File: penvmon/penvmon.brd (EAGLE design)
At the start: 91.9 x 100 mm, 19 parts, among them IC2 7805TV, U1 ZC563900

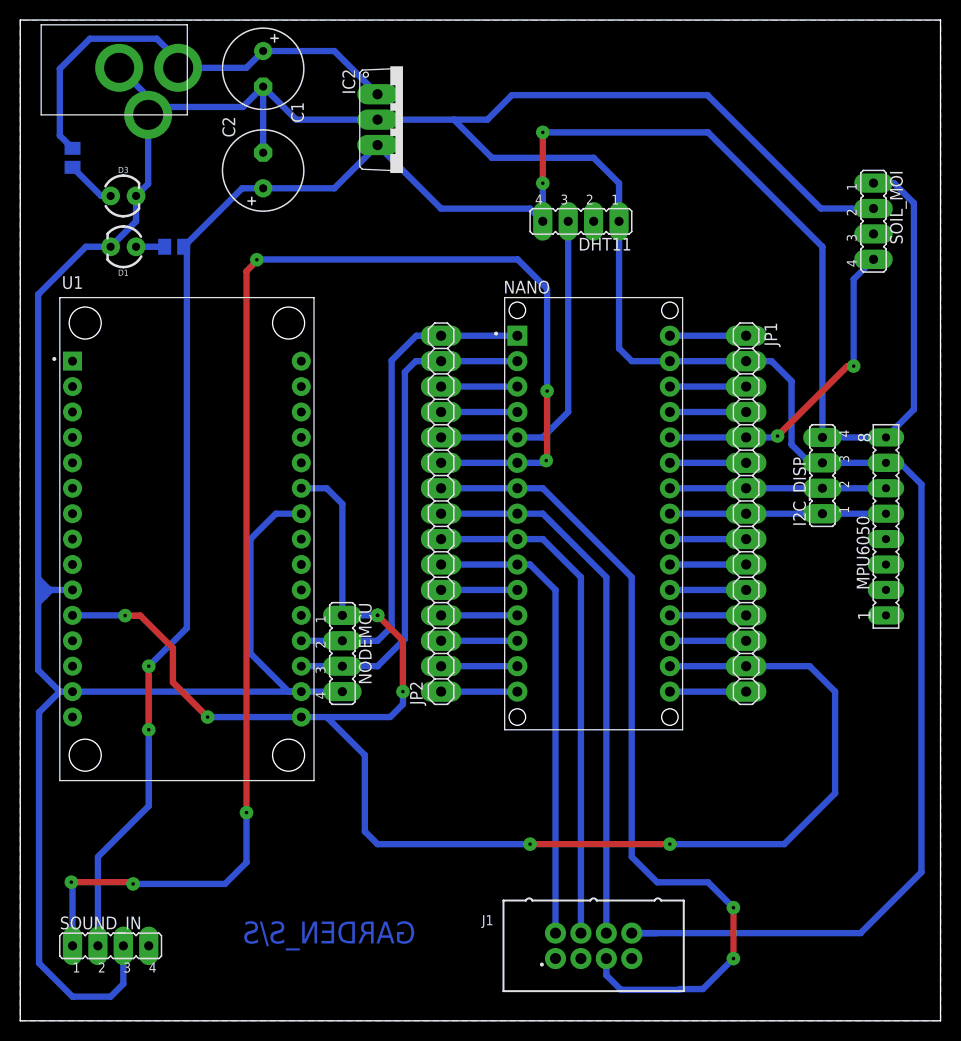
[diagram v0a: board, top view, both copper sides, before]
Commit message: added pcb image
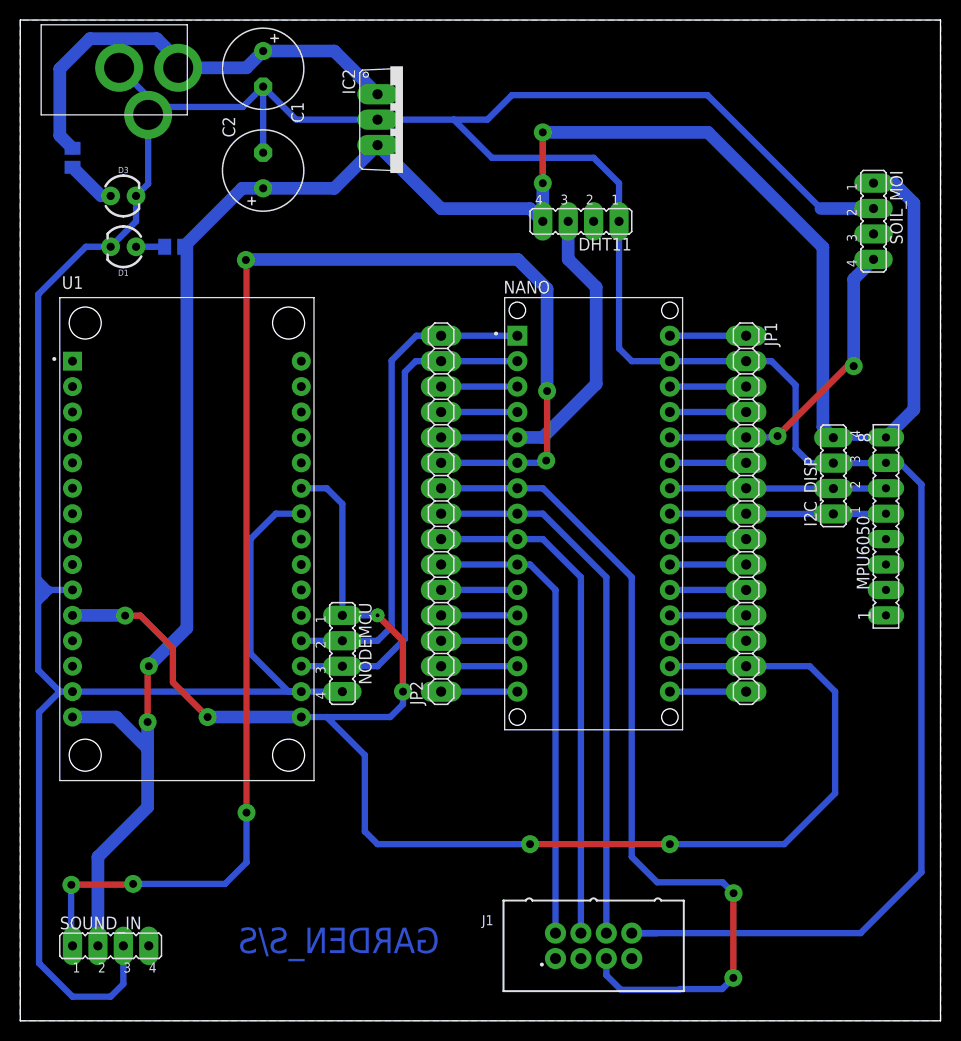
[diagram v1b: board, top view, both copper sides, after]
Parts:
- moved I2C_DISP 1.09 mm to (81.2, 54.5)
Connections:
- net 5V: now also U1.15
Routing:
- net 5V: track 213.4 -> 221.6 mm
- net DHT: track 32.8 -> 35.1 mm
- net LEFT: track 84.3 -> 86.3 mm
